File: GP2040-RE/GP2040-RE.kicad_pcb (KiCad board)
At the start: 4 copper layers, 63.2 x 36.1 mm, 52 parts, among them J1 I2C Target, J2 I2C Controller, J3 SM03B-SRSS-TB_LF__SN_, J4 USB Programming, J5 Conn_01x03, J6 microSD, J7 RJ-45, J8 Conn_01x10, Q1 NPN 65V 0.1A, U1 RP2040, U2 16M, U4 Linear Regulator, U5 TPS3702CX50DDCR

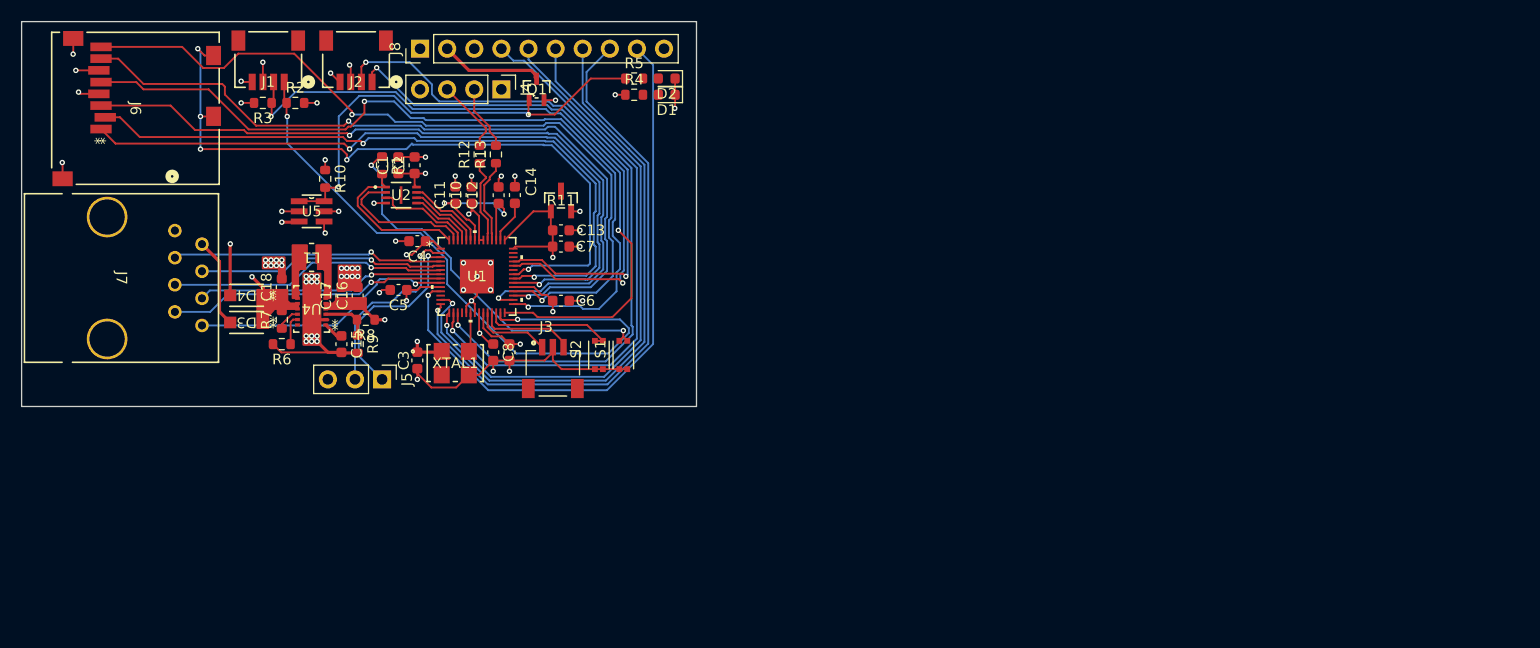
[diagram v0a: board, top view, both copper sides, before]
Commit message: What a roller coaster
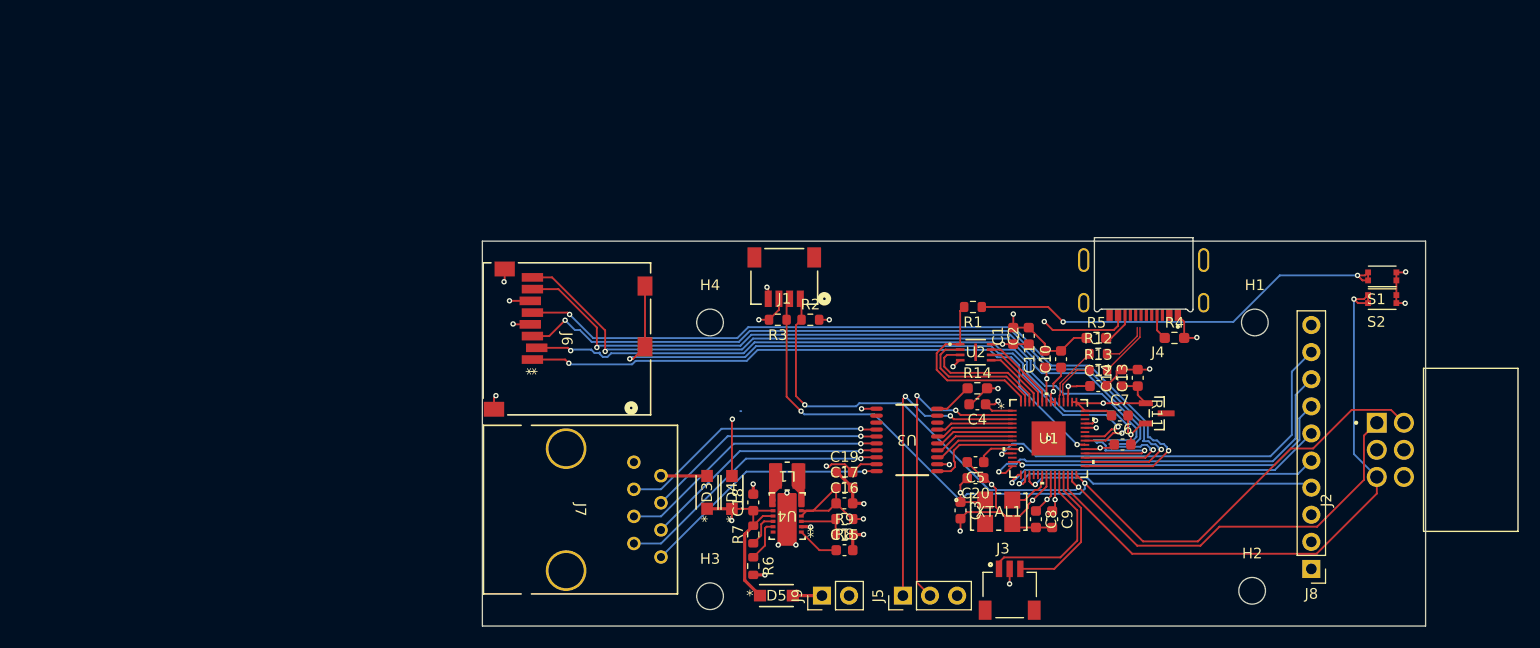
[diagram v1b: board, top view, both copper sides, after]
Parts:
- removed D1, D2: LED_Small, LED_SMD:LED_0603_1608Metric
- removed Q1: NPN 65V 0.1A, GP2040-RE:SOT-323-3_2P2X1P35_ONS
- removed R10: 10k, Resistor_SMD:R_0603_1608Metric
- removed U5: TPS3702CX50DDCR, GP2040-RE:DDC0006A_N
- added C19: 0.1uF, Capacitor_SMD:C_0603_1608Metric, F.Cu at (114.2, 90.2)
- added C20: 0.1uf, Capacitor_SMD:C_0603_1608Metric, F.Cu at (126.5, 90.8)
- added D5: 20V 1A, GP2040-RE:SDO_SOD-123FL_ONS, F.Cu at (107.8, 101.8)
- added H1: MountingHole, MountingHole:MountingHole_2.5mm, F.Cu at (152.7, 76.2)
- added H2: MountingHole, MountingHole:MountingHole_2.5mm, F.Cu at (152.4, 101.3)
- added H3: MountingHole, MountingHole:MountingHole_2.5mm, F.Cu at (101.6, 101.9)
- added H4: MountingHole, MountingHole:MountingHole_2.5mm, F.Cu at (101.6, 76.2)
- added J9: Conn_01x02, Connector_PinHeader_2.54mm:PinHeader_1x02_P2.54mm_Vertical, F.Cu at (112.1, 101.8)
- added R14: 130, Resistor_SMD:R_0603_1608Metric_Pad0.98x0.95mm_HandSolder, F.Cu at (126.7, 82.4)
- added U3: TXB0108PWR, GP2040-RE:TXB0108PWR, F.Cu at (120.0, 87.2)
- J2: value I2C Controller -> CONN HEADER R/A 6POS 2.54MM; footprint GP2040-RE:CONN_SM04B-SRSS-TB_JST -> GP2040-RE:WURTH_61200621721
- J4: value USB Programming -> GSB1C4621DS2HR; footprint Connector_PinHeader_2.54mm:PinHeader_1x04_P2.54mm_Vertical -> GP2040-RE:AMPHENOL_GSB1C4621DS2HR
- R4, R5: value 10k -> 5K1; footprint Resistor_SMD:R_0603_1608Metric -> Resistor_SMD:R_0603_1608Metric_Pad0.98x0.95mm_HandSolder
- moved J2 103.6 mm to (165.4, 88.1), turned to 90 degrees
- moved J8 96.7 mm to (157.9, 99.3), turned to 180 degrees
- moved S2 73.6 mm to (164.6, 74.0), turned to 180 degrees
- moved S1 71.5 mm to (164.6, 71.9), turned to 180 degrees
- moved J4 62.3 mm to (142.2, 70.4), turned to 180 degrees
- moved R12 60.9 mm to (138.0, 79.1), turned to 0 degrees
- moved R13 60.0 mm to (138.0, 80.7), turned to 0 degrees
- moved C1 59.8 mm to (130.0, 77.5)
- moved C2 59.7 mm to (131.5, 77.5)
- moved C14 59.4 mm to (140.2, 81.4)
- moved R11 59.3 mm to (143.5, 84.7), turned to -90 degrees
- moved C12 59.0 mm to (138.0, 82.2), turned to 0 degrees
- moved C10 57.3 mm to (134.5, 79.6)
- moved C11 57.3 mm to (133.0, 79.6)
- moved R1 56.9 mm to (126.2, 74.8), turned to 180 degrees
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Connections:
- J2 pad 1: /SDA_1 -> /SDA_0
- J2 pad 2: /SCL_1 -> /SCL_0
- J2 pad 5: (no net) -> /RUN
- J2 pad 6: (no net) -> VCC
- J8 pad 2: Net-(J8-Pin_2) -> +3.3V
- R4 pad 1: +3.3V -> Net-(J4-CC1)
- R4 pad 2: Net-(D1-A) -> GND
- R5 pad 1: /5V_EN -> GND
- R5 pad 2: Net-(D2-A) -> Net-(J4-CC2)
- U1 pad 4: /GreenStripe -> /3v3GreenStripe
- U1 pad 5: /BlueSolid -> /3v3BlueSolid
- U1 pad 6: /BlueStripe -> /3v3BlueStripe
- U1 pad 7: /GreenSolid -> /3v3GreenSolid
- U1 pad 8: /BrownStripe -> /3v3BrownStripe
- U1 pad 9: /BrownSolid -> /3v3BrownSolid
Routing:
- net VCC: track 0.00 -> 62.7 mm
- net /SCL_1: track 52.6 -> 1.11 mm, vias 2 -> 1
- net /SDA_1: track 50.5 -> 1.06 mm, vias 2 -> 1
- net /RUN: track 12.4 -> 58.0 mm, vias 0 -> 1
- net /5V_EN: track 42.7 -> 0.00 mm, vias 2 -> 0
- net /InputVoltage: track 10.1 -> 36.1 mm
- net /SPI1_SCK: track 56.7 -> 31.6 mm
- net /OCS: track 52.5 -> 27.8 mm
- net /RESET: track 52.7 -> 29.5 mm
- net /Data_Command: track 53.9 -> 31.2 mm
- net /SPI1_TX_MOSI: track 57.1 -> 37.0 mm
- net /SPI1_RX_MISO: track 58.1 -> 38.4 mm
- net /SDA_0: track 61.6 -> 78.7 mm
- net /SCL_0: track 65.2 -> 81.0 mm
- net /UART_RX: track 18.3 -> 29.7 mm, vias 1 -> 2
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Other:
- board size 63.2 x 36.1 mm -> 88.4 x 36.1 mm
